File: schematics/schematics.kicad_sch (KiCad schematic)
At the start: 4 parts, among them U1 SFH617A-1X001, U2 SFH617A-1X001, U3 MAX232

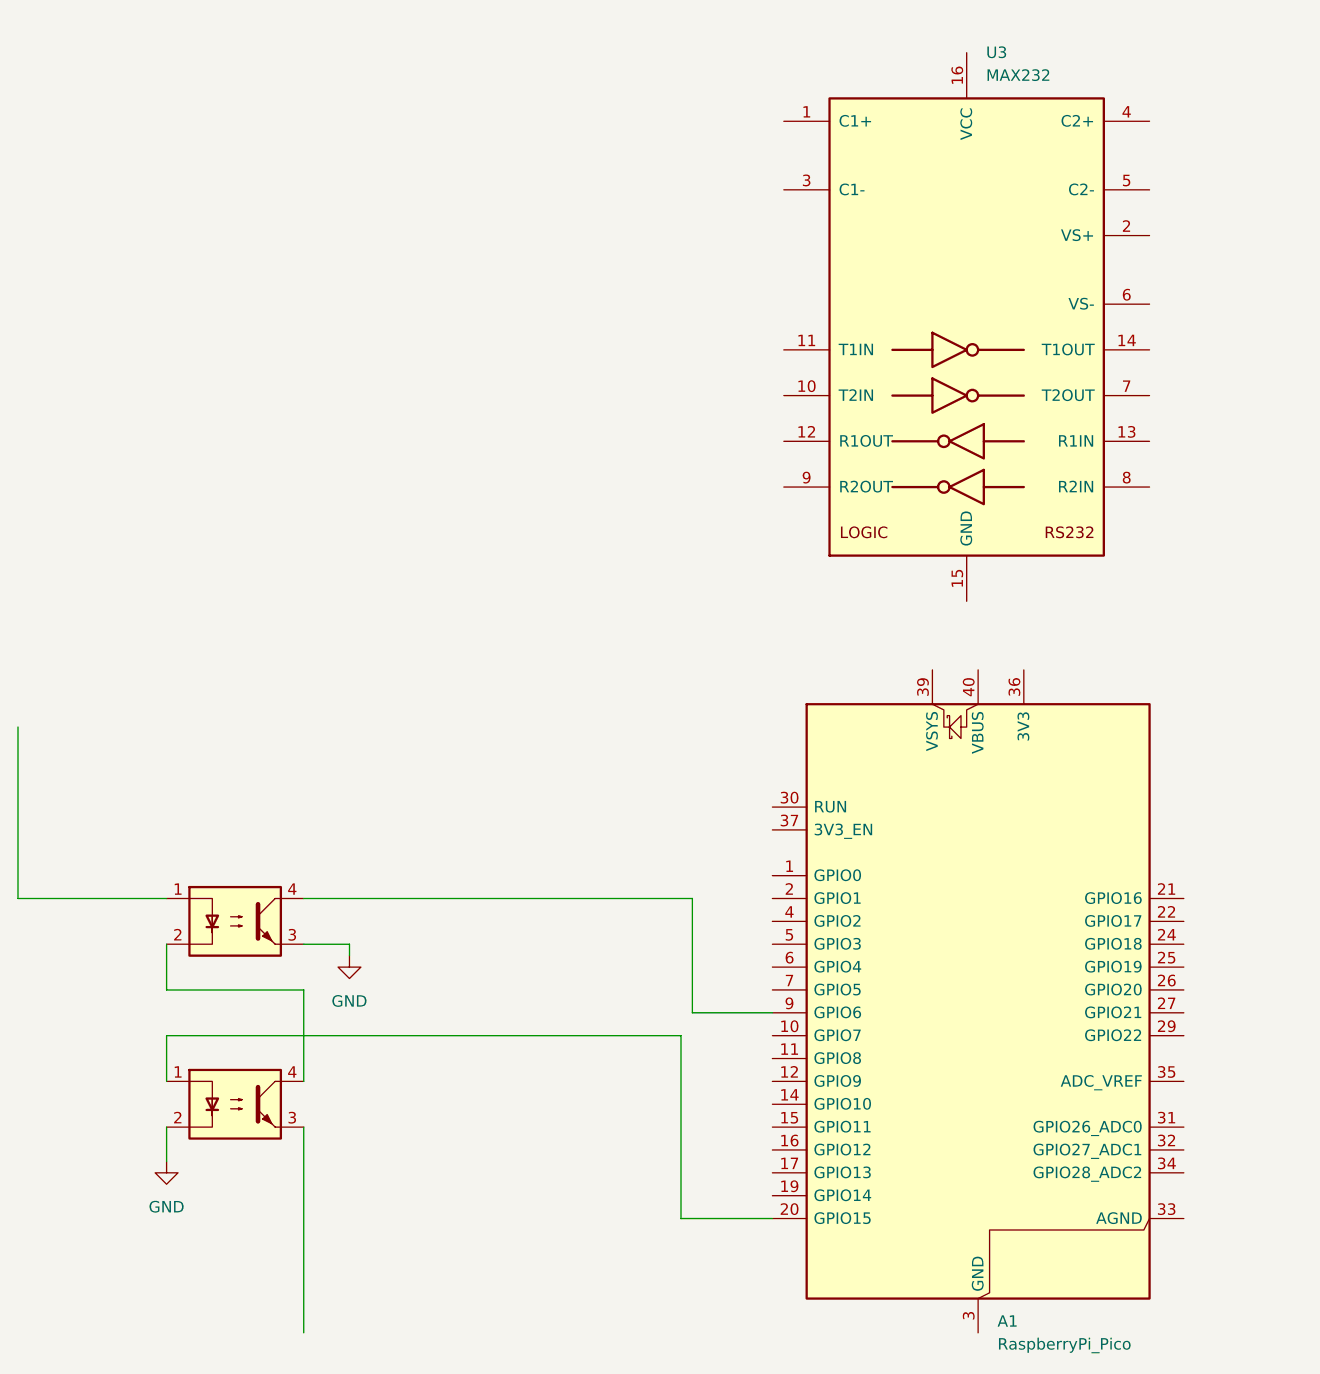
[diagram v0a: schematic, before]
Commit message: finish schematics
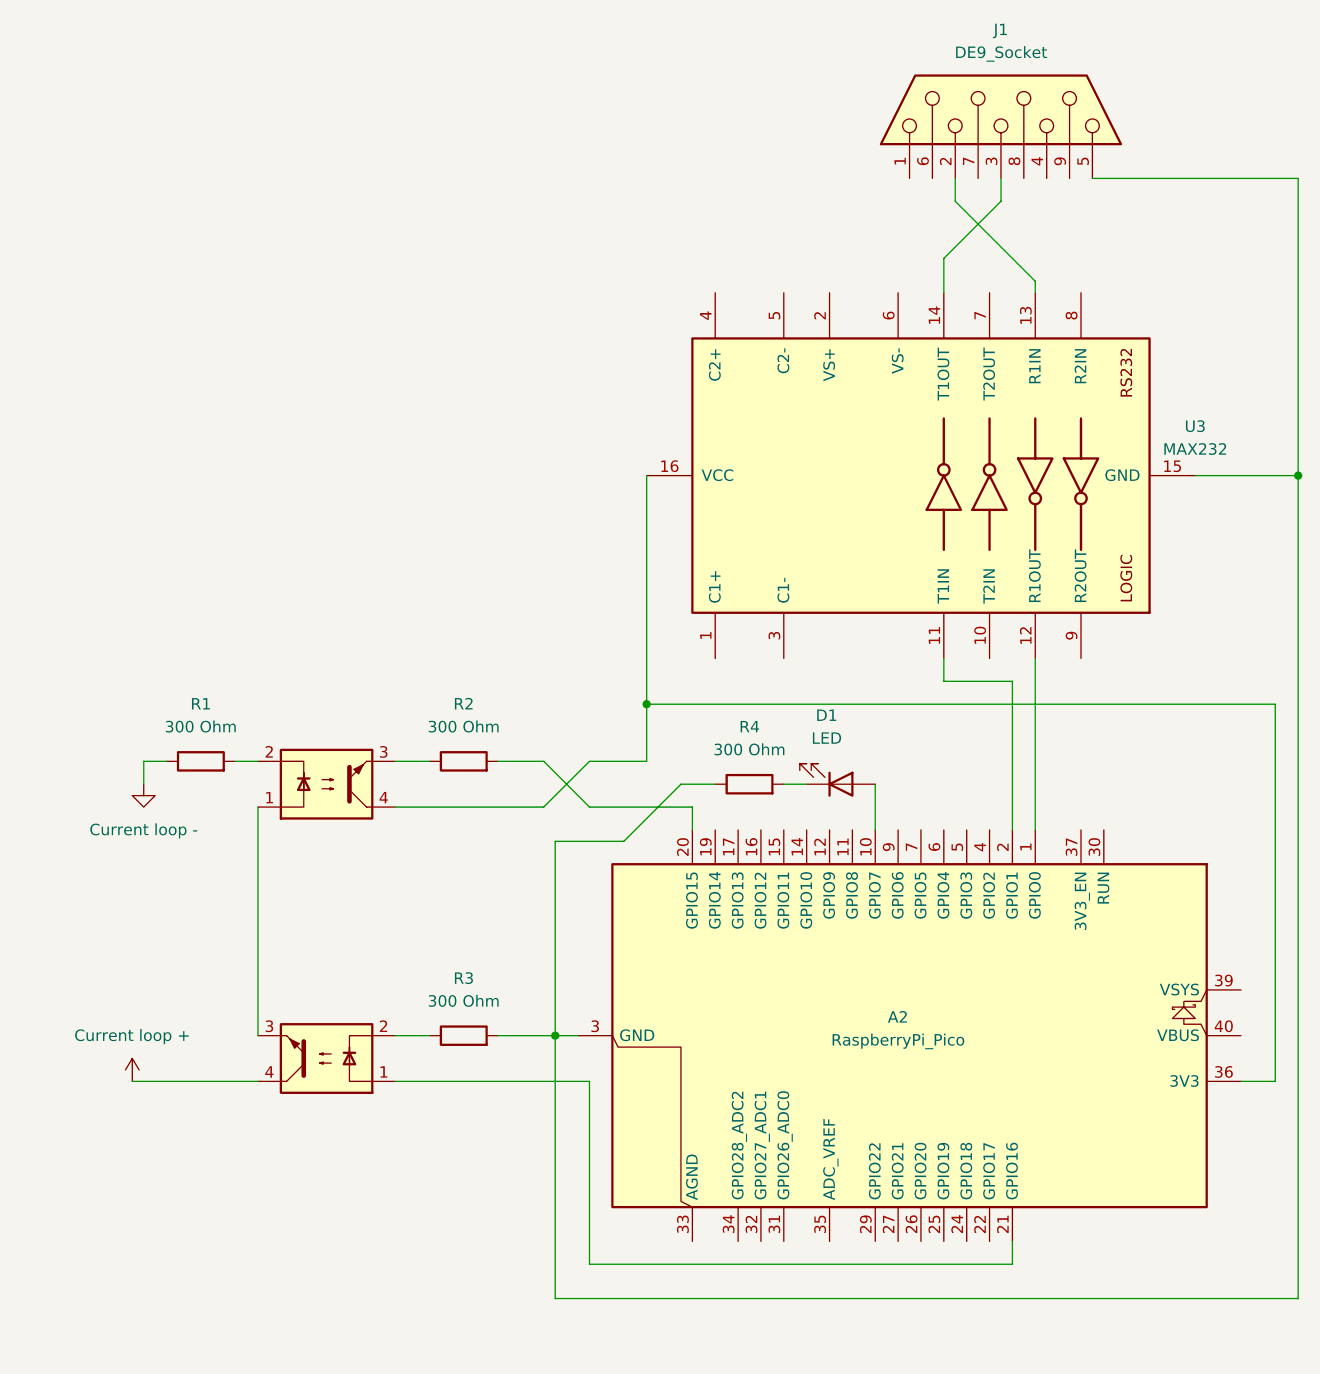
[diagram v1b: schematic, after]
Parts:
- removed A1: RaspberryPi_Pico, Module:RaspberryPi_Pico_Common_Unspecified, symbol MCU_Module:RaspberryPi_Pico
- removed U1, U2: SFH617A-1X001, Package_DIP:DIP-4_W7.62mm, symbol Isolator:SFH617A-1X001
- added A2: RaspberryPi_Pico, Module:RaspberryPi_Pico_Common_Unspecified, symbol MCU_Module:RaspberryPi_Pico
- added D1: LED, symbol Device:LED
- added J1: DE9_Socket, symbol Connector:DE9_Socket
- added R1, R2, R3, R4: 300 Ohm, symbol Device:R
- added U4, U5: SFH617A-1X001, Package_DIP:DIP-4_W7.62mm, symbol Isolator:SFH617A-1X001
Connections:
- net at U3.11 (T1IN): now also A2.2 (GPIO1)
- net at U3.12 (R1OUT): now also A2.1 (GPIO0)
- net at U3.13 (R1IN): now also J1.2
- net at U3.14 (T1OUT): now also J1.3
- net at U3.15 (GND): now also A2.13 (GND), A2.18 (GND), A2.23 (GND), A2.28 (GND), A2.3 (GND), A2.38 (GND), A2.8 (GND), J1.5, R3.2, R4.1
- net at U3.16 (VCC): now also A2.36 (3V3), U5.4
- new net: A2.21 (GPIO16), U4.1
- new net: R3.1, U4.2
- new net: U4.3, U5.1
- new net: D1.1 (K), R4.2
- new net: A2.10 (GPIO7), D1.2 (A)
- new net: A2.20 (GPIO15), R2.2
- new net: R1.2, U5.2
- new net: R2.1, U5.3
- new net Current loop +: U4.4
- new net Current loop -: R1.1
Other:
- moved on the sheet: U3
